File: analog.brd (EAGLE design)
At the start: 160 x 100 mm, 42 parts, among them IC1 NE555, Q1 BC548A, T1 BTV58, T2 BTV58

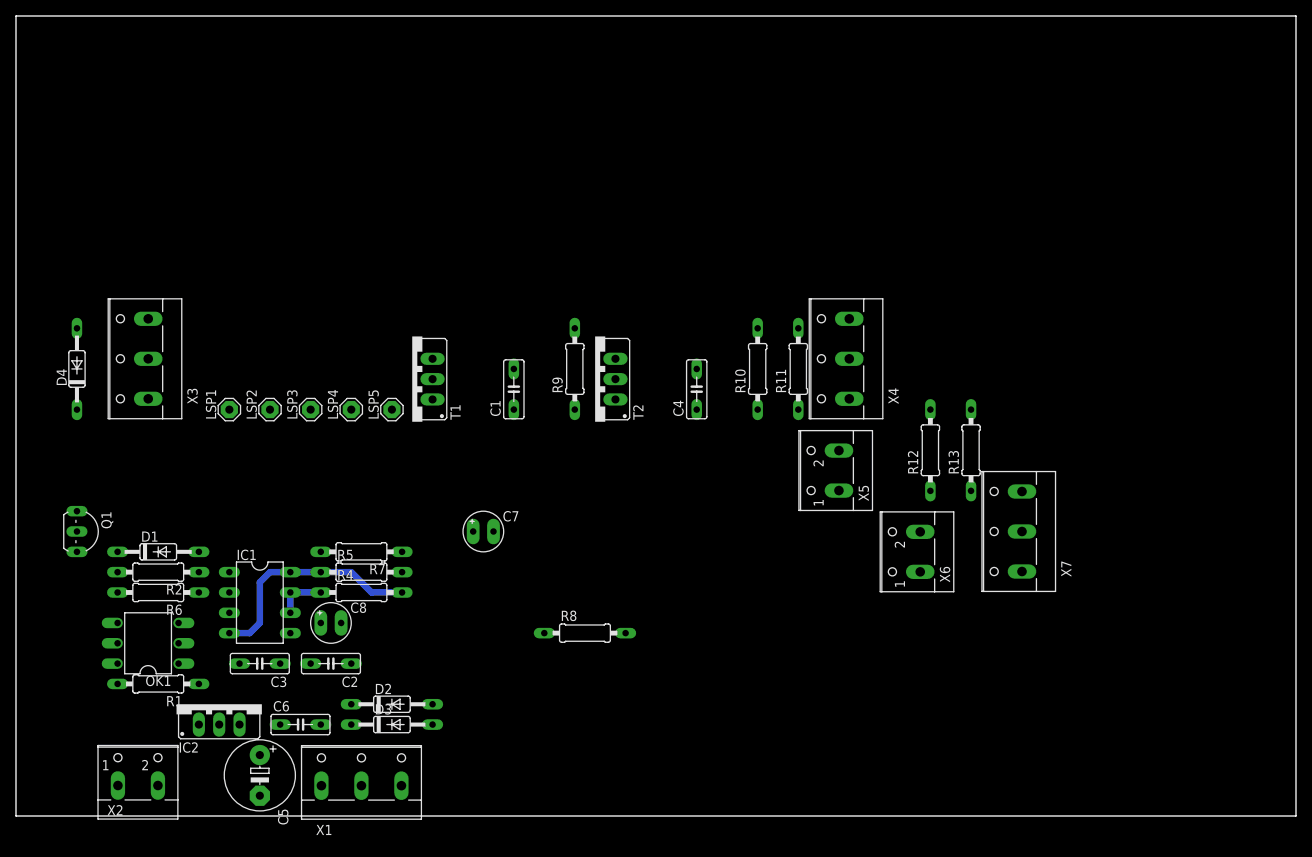
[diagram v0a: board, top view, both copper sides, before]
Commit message: routing
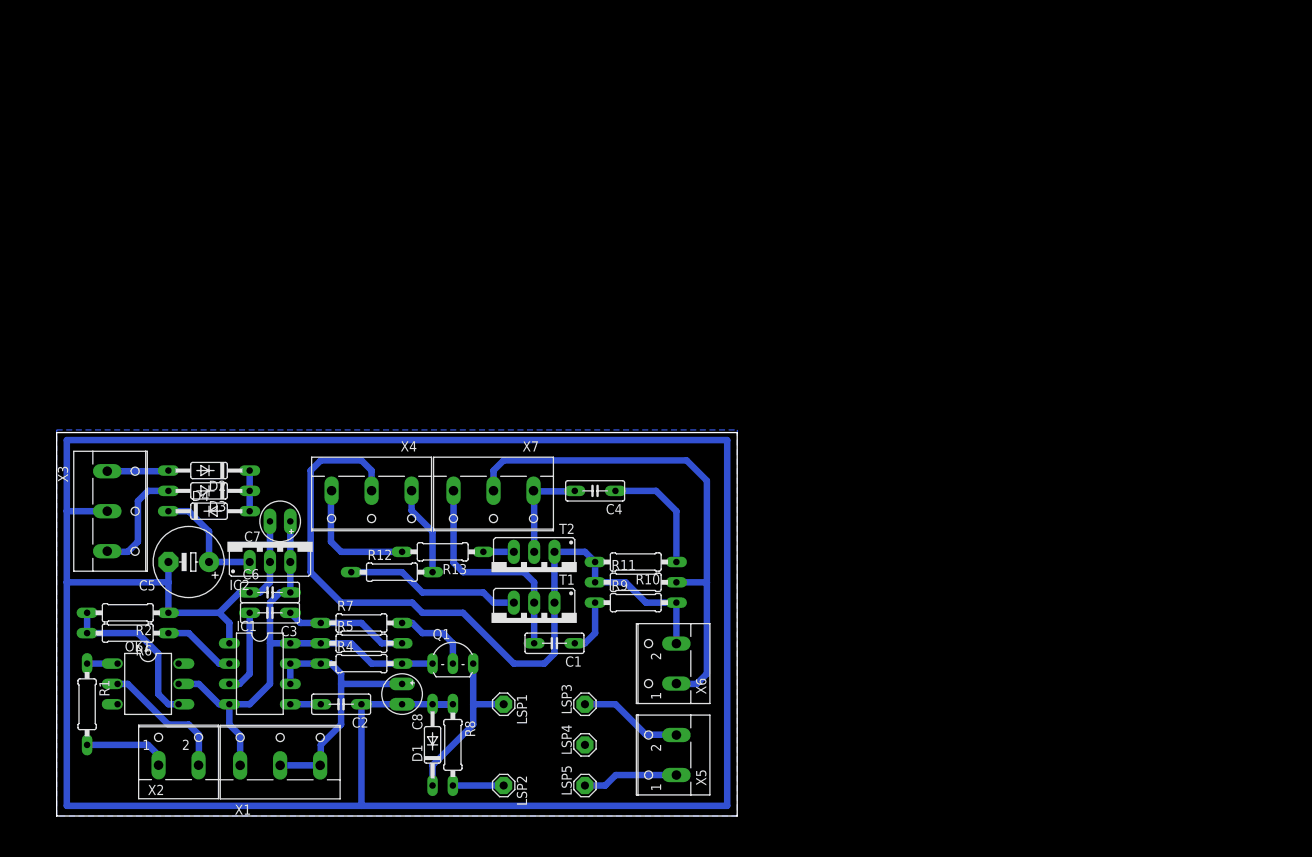
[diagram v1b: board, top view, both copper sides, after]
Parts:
- moved R12 69.0 mm to (47.0, 30.5), turned to 0 degrees
- moved R13 67.3 mm to (53.3, 33.0), turned to 180 degrees
- moved X7 64.9 mm to (59.7, 39.4), turned to 180 degrees
- moved X4 61.1 mm to (44.5, 39.4), turned to 180 degrees
- moved LSP2 55.3 mm to (61.0, 3.81), turned to 270 degrees
- moved LSP5 52.8 mm to (71.1, 3.81)
- moved LSP4 51.1 mm to (71.1, 8.89)
- moved LSP3 50.3 mm to (71.1, 14.0)
- moved LSP1 50.3 mm to (61.0, 14.0), turned to 270 degrees
- moved Q1 48.2 mm to (54.6, 20.3), turned to 0 degrees
- moved D1 41.9 mm to (52.1, 8.89), turned to 90 degrees
- moved X5 41.0 mm to (81.3, 7.62)
- moved D2 37.1 mm to (24.1, 43.2), turned to 180 degrees
- moved D3 37.1 mm to (24.1, 40.6), turned to 180 degrees
- moved T1 34.1 mm to (64.8, 24.1), turned to 180 degrees
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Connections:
- new net N$27: R10.2, R11.1, R9.2, T1.C, T2.C, X4.2, X6.2
- net GND: no longer R11.2, X6.1
- net N$21: now also R11.2, X6.1; no longer R10.2, R11.1, R9.2, T1.C, T2.C, X4.2, X6.2
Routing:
- net GND: track 0.00 -> 333.6 mm
- net N$27: track 0.00 -> 96.8 mm
- net N$21: track 0.00 -> 63.1 mm
- net VCC: track 28.8 -> 65.2 mm
- net N$5: track 6.35 -> 34.6 mm
- net N$20: track 0.00 -> 27.7 mm
- net N$25: track 0.00 -> 21.9 mm
- net N$9: track 0.00 -> 21.2 mm
- net N$2: track 0.00 -> 20.6 mm
- net N$14: track 0.00 -> 16.6 mm
- net N$24: track 0.00 -> 15.9 mm
- net N$6: track 0.00 -> 15.5 mm
- net +12V: track 0.00 -> 15.0 mm
- net N$22: track 0.00 -> 15.0 mm
- net N$13: track 0.00 -> 13.8 mm
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- added copper zone on layer 16, net GND
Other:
- board size 160 x 100 mm -> 85.1 x 47.9 mm
